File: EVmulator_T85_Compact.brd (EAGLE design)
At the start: 23 x 13 mm, 24 parts, among them Q2 DMN3404L-7, U1 ATTINY85V

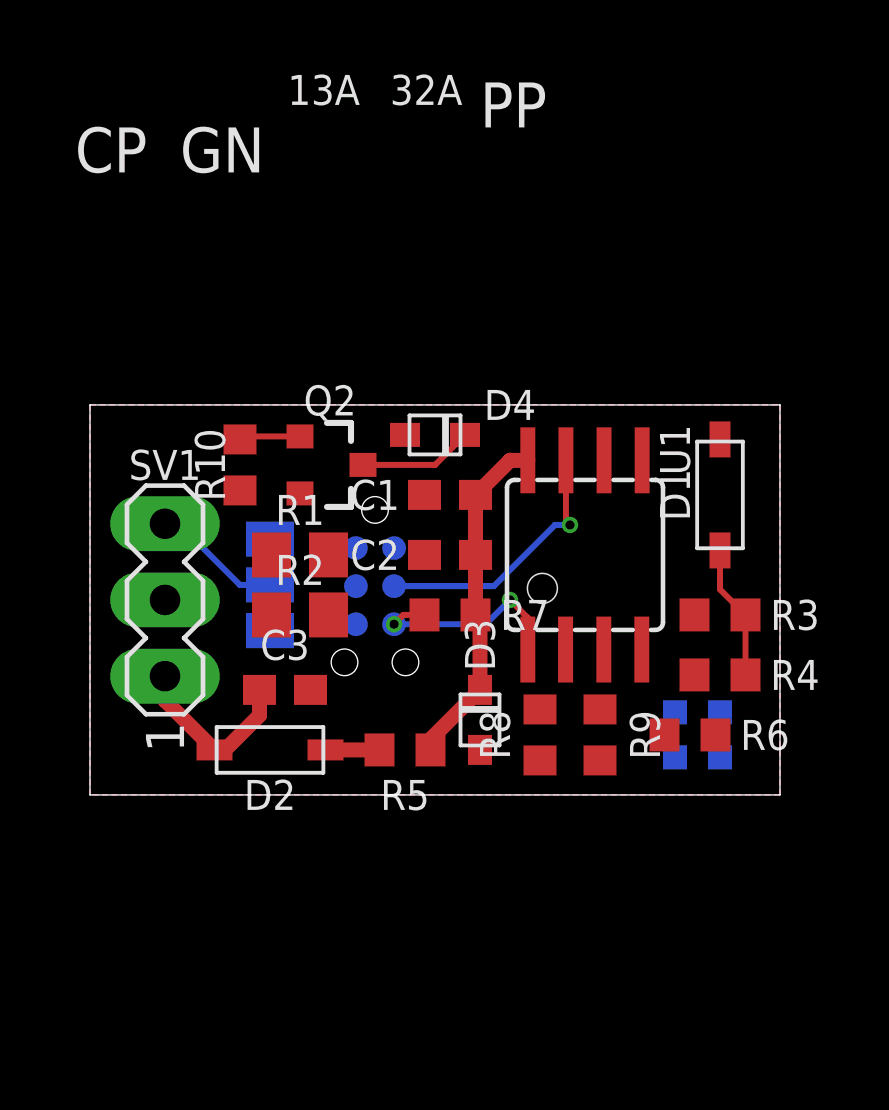
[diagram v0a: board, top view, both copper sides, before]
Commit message: Finished compact version
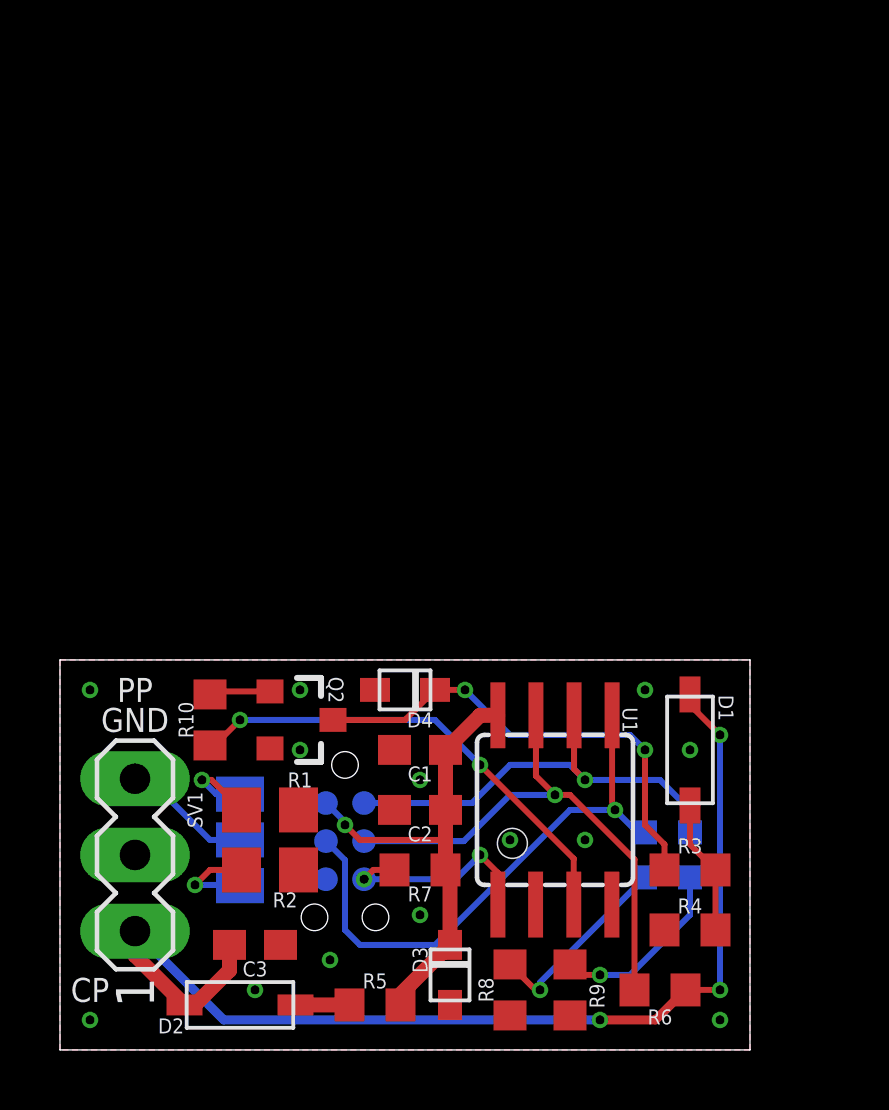
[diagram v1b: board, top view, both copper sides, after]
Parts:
- moved C1 8.56 mm to (12.0, 10.0)
- moved C2 8.56 mm to (12.0, 8.00)
- moved C3 8.56 mm to (6.50, 3.50)
- moved D1 8.56 mm to (21.0, 10.0)
- moved D2 8.56 mm to (6.00, 1.50)
- moved D3 8.56 mm to (13.0, 2.50)
- moved D4 8.56 mm to (11.5, 12.0)
- moved J1 8.56 mm to (9.50, 9.50)
- moved Q2 8.56 mm to (8.00, 11.0)
- moved R1 8.56 mm to (7.00, 8.00)
- moved R10 8.56 mm to (5.00, 11.0)
- moved R2 8.56 mm to (7.00, 6.00)
- moved R3 8.56 mm to (21.0, 6.00)
- moved R4 8.56 mm to (21.0, 4.00)
- moved R5 8.56 mm to (10.5, 1.50)
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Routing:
- net CON_CP: track 5.97 -> 37.4 mm, vias 0 -> 3
- net LED_GN: track 0.00 -> 18.9 mm, vias 0 -> 1
- net N$10: track 0.00 -> 15.9 mm, vias 0 -> 2
- net LED_RD: track 0.00 -> 15.1 mm, vias 0 -> 1
- net N$5: track 3.81 -> 15.9 mm, vias 0 -> 2
- net PWM_DET: track 8.92 -> 17.8 mm
- net N$3: track 0.00 -> 6.55 mm, vias 0 -> 1
- net N$4: track 0.00 -> 6.37 mm, vias 0 -> 1
- net 4V7: track 11.5 -> 16.0 mm, vias 0 -> 1
- net N$1: track 0.00 -> 3.52 mm, vias 0 -> 1
- net N$2: track 0.00 -> 3.27 mm, vias 0 -> 1
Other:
- board text added: "25A"
- board text added: "GND"
- board text removed: "32A"
- board text removed: "GN"
